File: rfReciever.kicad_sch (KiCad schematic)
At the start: 27 parts, among them P1 USB_C_Plug_USB2.0, SW1 SW_Push, SW2 SW_Push, U1 XBee_SMT, U2 CP2102N-Axx-xQFN20, U3 USBLC6-2SC6

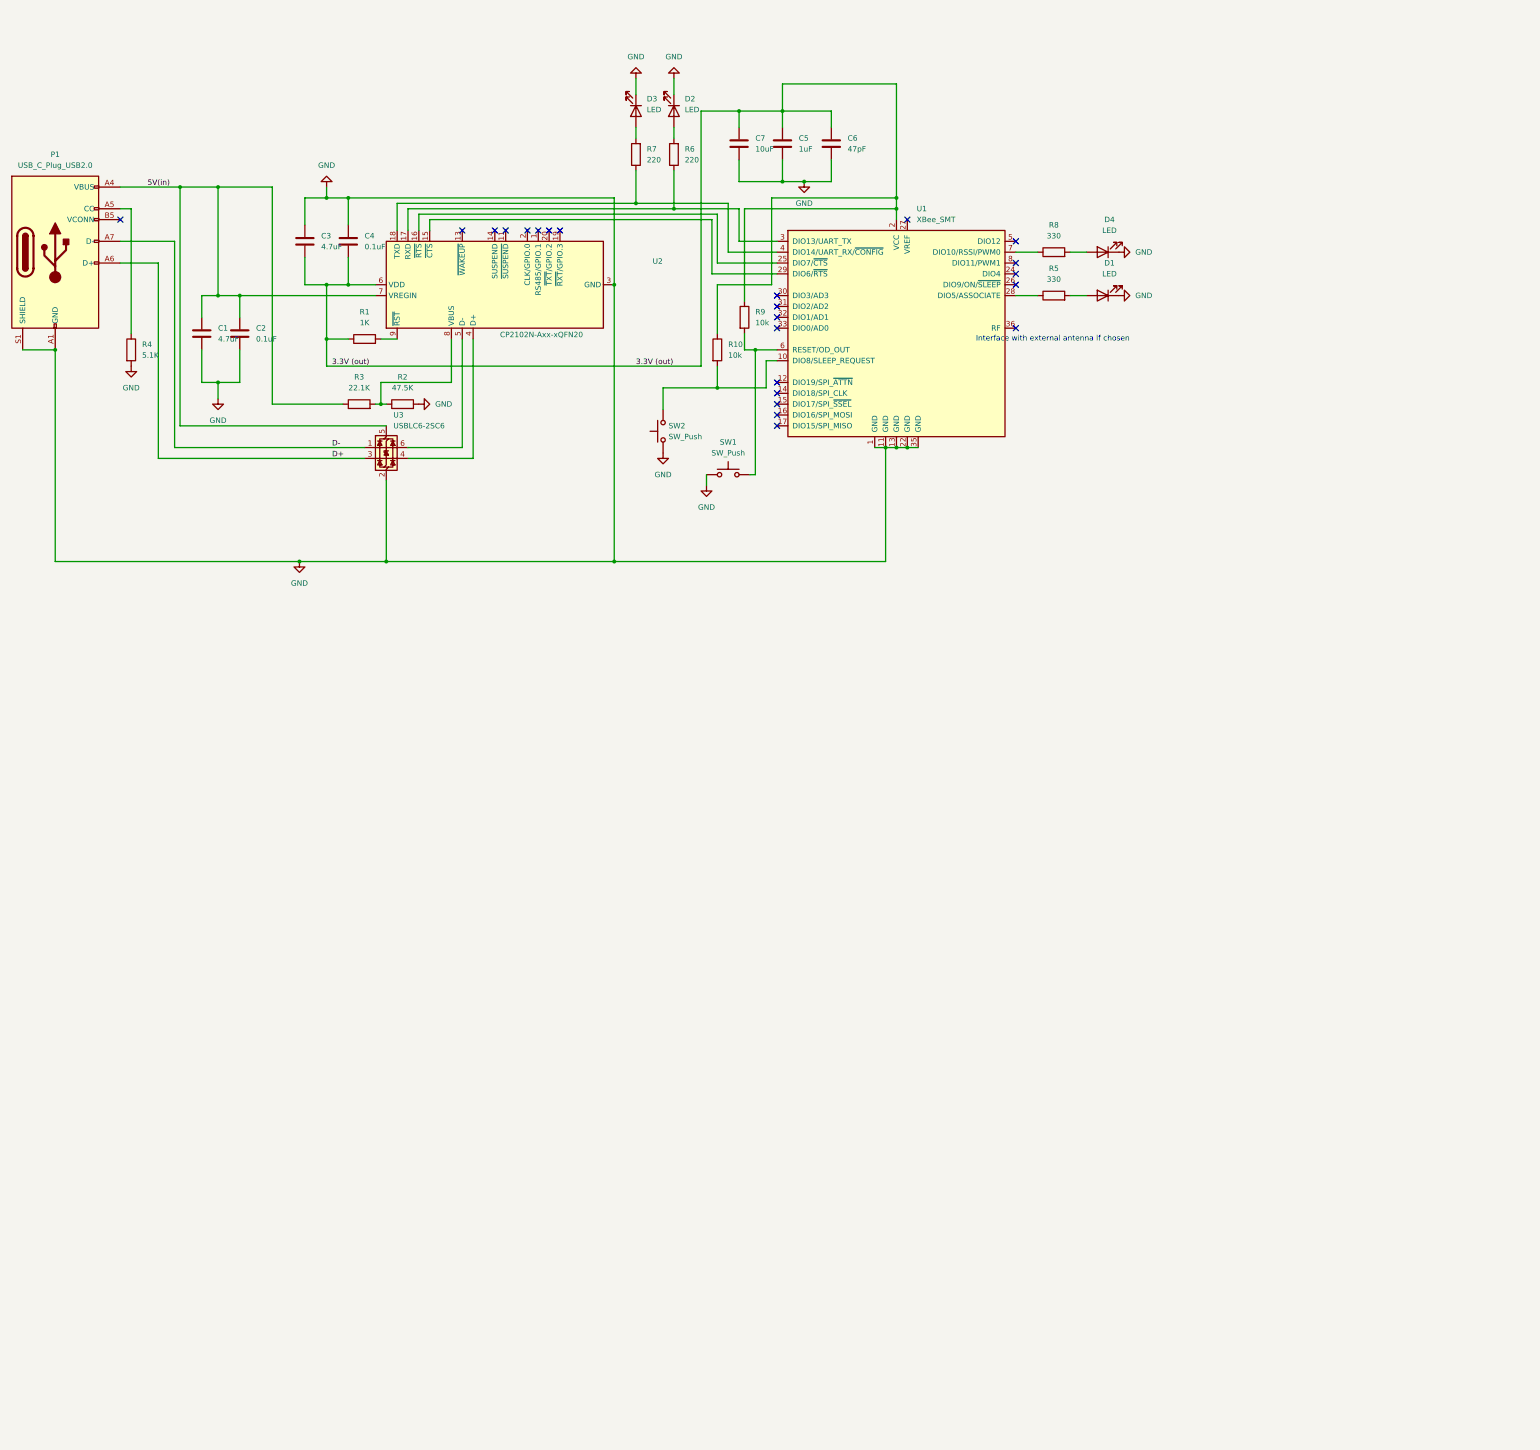
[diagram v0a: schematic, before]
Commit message: double schematic about to fix
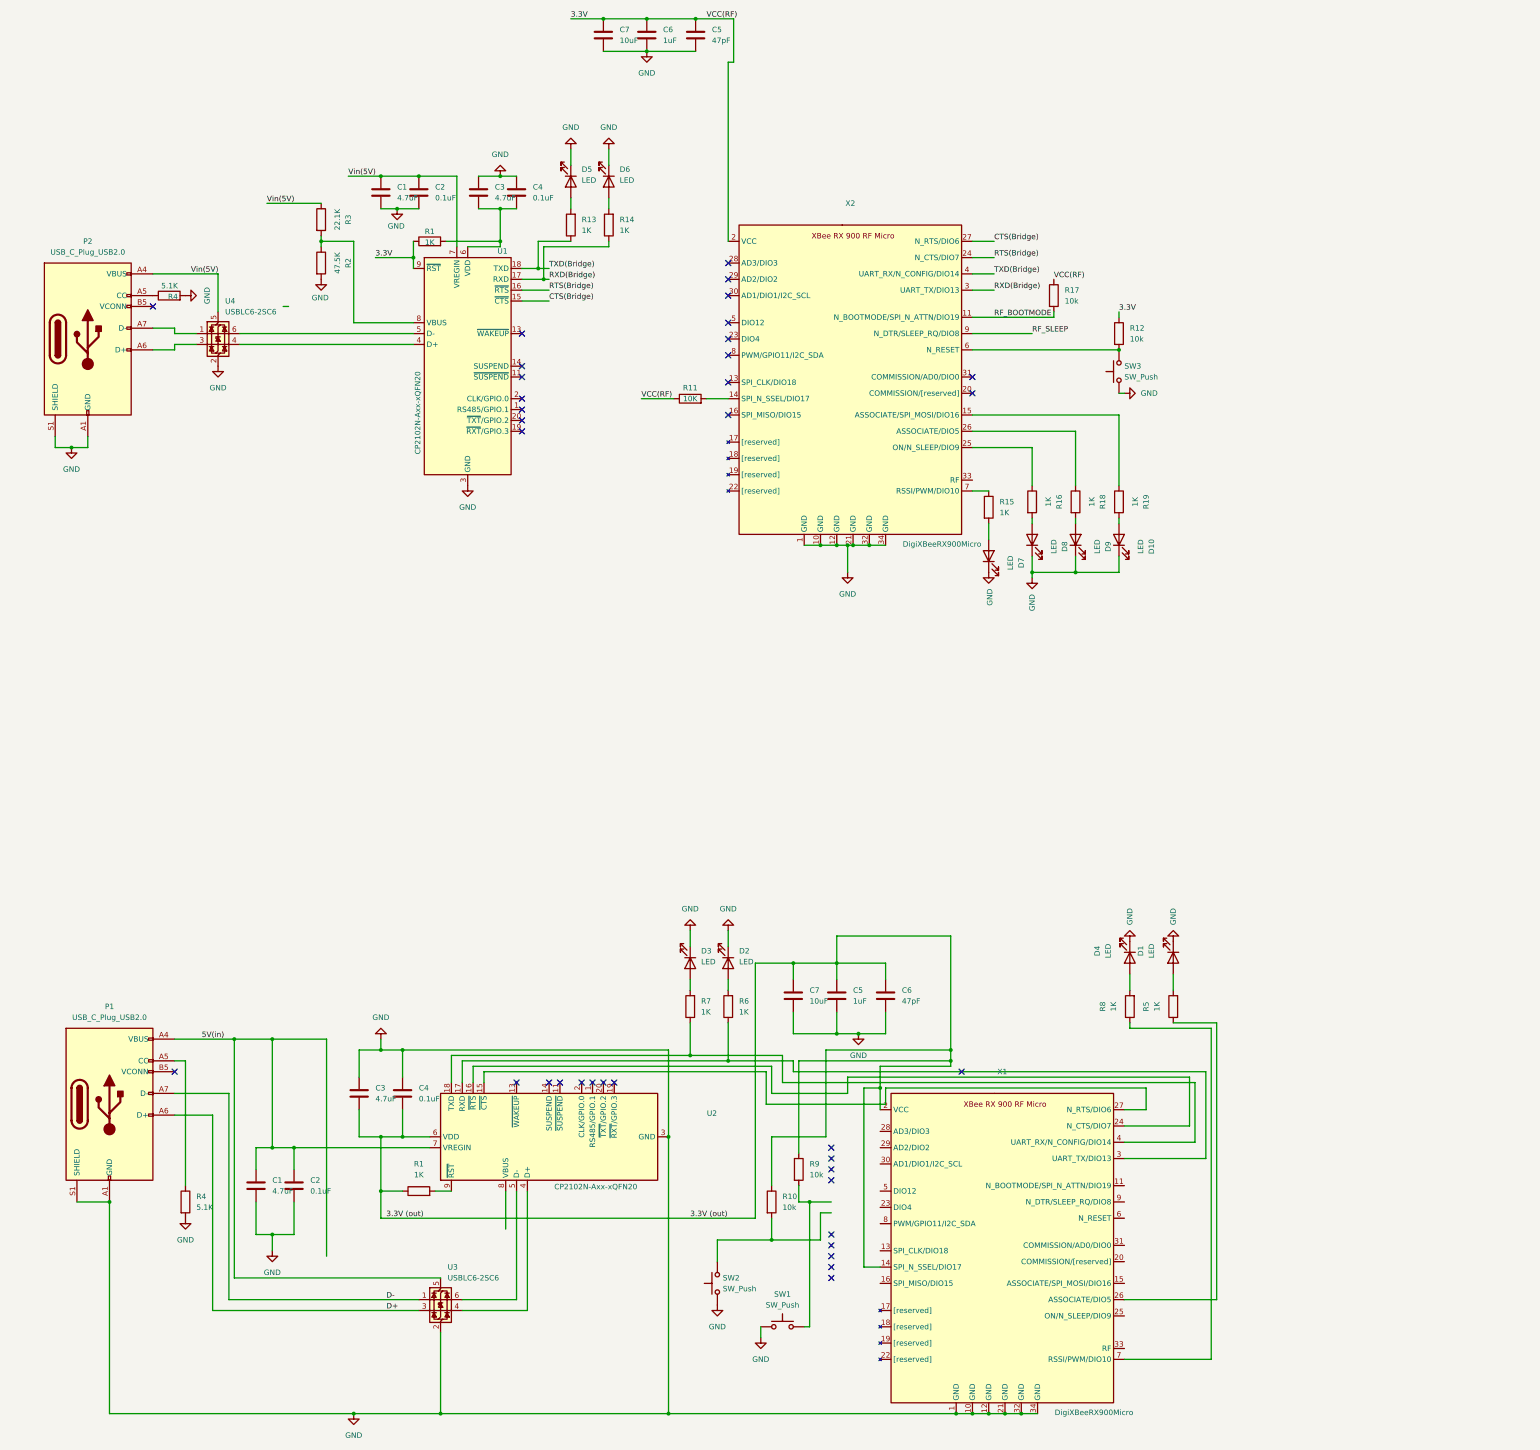
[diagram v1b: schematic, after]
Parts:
- removed U1: XBee_SMT, RF_Module:Digi_XBee_SMT, symbol RF_ZigBee:XBee_SMT
- added C1, C3: 4.7uF, Capacitor_SMD:C_0805_2012Metric, symbol Device:C
- added C2, C4: 0.1uF, Capacitor_SMD:C_0805_2012Metric, symbol Device:C
- added C5: 47pF, Capacitor_SMD:C_0805_2012Metric, symbol Device:C
- added C6: 1uF, Capacitor_SMD:C_0805_2012Metric, symbol Device:C
- added C7: 10uF, Capacitor_SMD:C_0805_2012Metric, symbol Device:C
- added D10, D5, D6, D7, D8, D9: LED, LED_SMD:LED_0805_2012Metric, symbol Device:LED
- added P2: USB_C_Plug_USB2.0, Connector_USB:USB_C_Plug_JAE_DX07P024AJ1, symbol Connector:USB_C_Plug_USB2.0
- added R1, R13, R14, R15, R16, R18, R19: 1K, Resistor_SMD:R_0805_2012Metric, symbol Device:R
- added R11: 10K, Resistor_SMD:R_0805_2012Metric, symbol Device:R
- added R12, R17: 10k, Resistor_SMD:R_0805_2012Metric, symbol Device:R
- added R4: 5.1K, Resistor_SMD:R_0805_2012Metric, symbol Device:R
- added SW3: SW_Push, Button_Switch_THT:SW_PUSH_6mm_H4.3mm, symbol Switch:SW_Push
- added U1: CP2102N-Axx-xQFN20, Audio_Module:QFN24_CP2102N_SIL, symbol Interface_USB:CP2102N-Axx-xQFN20
- added U4: USBLC6-2SC6, Package_TO_SOT_SMD:SOT-23-6, symbol Power_Protection:USBLC6-2SC6
- added X1, X2: DigiXBeeRX900Micro, symbol DataAcqLeaderBoard-Symbols:DigiXBeeRX900Micro
- C1, C3, C5: footprint Capacitor_SMD:C_0603_1608Metric_Pad1.08x0.95mm_HandSolder -> Capacitor_SMD:C_0805_2012Metric
- C2: footprint Capacitor_SMD:C_01005_0402Metric_Pad0.57x0.30mm_HandSolder -> Capacitor_SMD:C_0805_2012Metric
- C4, C6: footprint Capacitor_SMD:C_0402_1005Metric_Pad0.74x0.62mm_HandSolder -> Capacitor_SMD:C_0805_2012Metric
- C7: footprint Capacitor_SMD:C_0805_2012Metric_Pad1.18x1.45mm_HandSolder -> Capacitor_SMD:C_0805_2012Metric
- D1, D4: footprint LED_SMD:LED_0201_0603Metric -> LED_SMD:LED_0805_2012Metric
- D2, D3: footprint LED_SMD:LED_0603_1608Metric_Pad1.05x0.95mm_HandSolder -> LED_SMD:LED_0805_2012Metric
- R1, R10, R2, R3, R4, R9: footprint Resistor_SMD:R_0603_1608Metric_Pad0.98x0.95mm_HandSolder -> Resistor_SMD:R_0805_2012Metric
- R5, R8: value 330 -> 1K; footprint Resistor_SMD:R_0603_1608Metric_Pad0.98x0.95mm_HandSolder -> Resistor_SMD:R_0805_2012Metric
- R6, R7: value 220 -> 1K; footprint Resistor_SMD:R_0603_1608Metric_Pad0.98x0.95mm_HandSolder -> Resistor_SMD:R_0805_2012Metric
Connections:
- net 3.3V (out): now also X1.14 (SPI_N_SSEL/DIO17), X1.2 (VCC)
- net 5V(in): no longer R3.1
- net GND: now also C1.2, C2.2, C3.1, C4.1, C5.2, C6.2, C7.2, D10.1 (K), D5.1 (K), D6.1 (K), D7.1 (K), D8.1 (K), D9.1 (K), P2.A1 (GND), P2.A12 (GND), P2.B1 (GND), P2.B12 (GND), P2.S1 (SHIELD), R4.2, SW3.1, U1.12 (GND), U1.21 (GND), U1.3 (GND), U4.2 (GND), X1.1 (GND), X1.10 (GND), X1.12 (GND), X1.21 (GND), X1.32 (GND), X1.34 (GND), X2.1 (GND), X2.10 (GND), X2.12 (GND), X2.21 (GND), X2.32 (GND), X2.34 (GND)
- net at R2.1, R3.2: now also U1.8 (VBUS); no longer U2.8 (VBUS)
- net at R7.1, U2.18 (TXD): now also X1.4 (UART_RX/N_CONFIG/DIO14)
- net at R6.1, U2.17 (RXD): now also X1.3 (UART_TX/DIO13)
- net at R8.1: now also X1.7 (RSSI/PWM/DIO10)
- net at R5.1: now also X1.26 (ASSOCIATE/DIO5)
- net at U2.16 (~{RTS}): now also X1.24 (N_CTS/DIO7)
- net at U2.15 (~{CTS}): now also X1.27 (N_RTS/DIO6)
- new net: D6.2 (A), R14.2
- new net: C3.2, C4.2, R1.2, U1.6 (VDD)
- new net: P2.A5 (CC), R4.1
- new net: R19.1, X2.15 (ASSOCIATE/SPI_MOSI/DIO16)
- new net: D10.2 (A), R19.2
- new net: R12.2, SW3.2, X2.6 (N_RESET)
- new net: R11.2, X2.14 (SPI_N_SSEL/DIO17)
- new net: D5.2 (A), R13.2
- new net: R16.1, X2.25 (ON/N_SLEEP/DIO9)
- new net: R18.1, X2.26 (ASSOCIATE/DIO5)
- new net: R15.1, X2.7 (RSSI/PWM/DIO10)
- new net: D7.2 (A), R15.2
- new net: D8.2 (A), R16.2
- new net: D9.2 (A), R18.2
- new net: P2.A6 (D+), U4.3 (I/O2)
- new net: P2.A7 (D-), U4.1 (I/O1)
- new net: U1.4 (D+), U4.4 (I/O2)
- new net: U1.5 (D-), U4.6 (I/O1)
- new net 3.3V: C5.1, C6.1, C7.1, R1.1, R11.1, R12.1, R17.1, U1.9 (~{RST}), X2.2 (VCC)
- new net CTS(Bridge): U1.15 (~{CTS}), X2.27 (N_RTS/DIO6)
- new net RF_BOOTMODE: R17.2, X2.11 (N_BOOTMODE/SPI_N_ATTN/DIO19)
- new net RF_SLEEP: X2.9 (N_DTR/SLEEP_RQ/DIO8)
- new net RTS(Bridge): U1.16 (~{RTS}), X2.24 (N_CTS/DIO7)
- new net RXD(Bridge): R14.1, U1.17 (RXD), X2.3 (UART_TX/DIO13)
- new net TXD(Bridge): R13.1, U1.18 (TXD), X2.4 (UART_RX/N_CONFIG/DIO14)
- new net Vin(5V): C1.1, C2.1, P2.A4 (VBUS), P2.A9 (VBUS), P2.B4 (VBUS), P2.B9 (VBUS), R3.1, U1.7 (VREGIN), U4.5 (VBUS)
- no-connect marks 23 -> 36
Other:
- note removed: "Interface with external antenna if chosen"
- moved on the sheet: C1, C2, C3, C4, C5, C6, C7, D1, D2, D3, D4, P1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

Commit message: Final Schematic preliminary pcb layout(pre-routing)
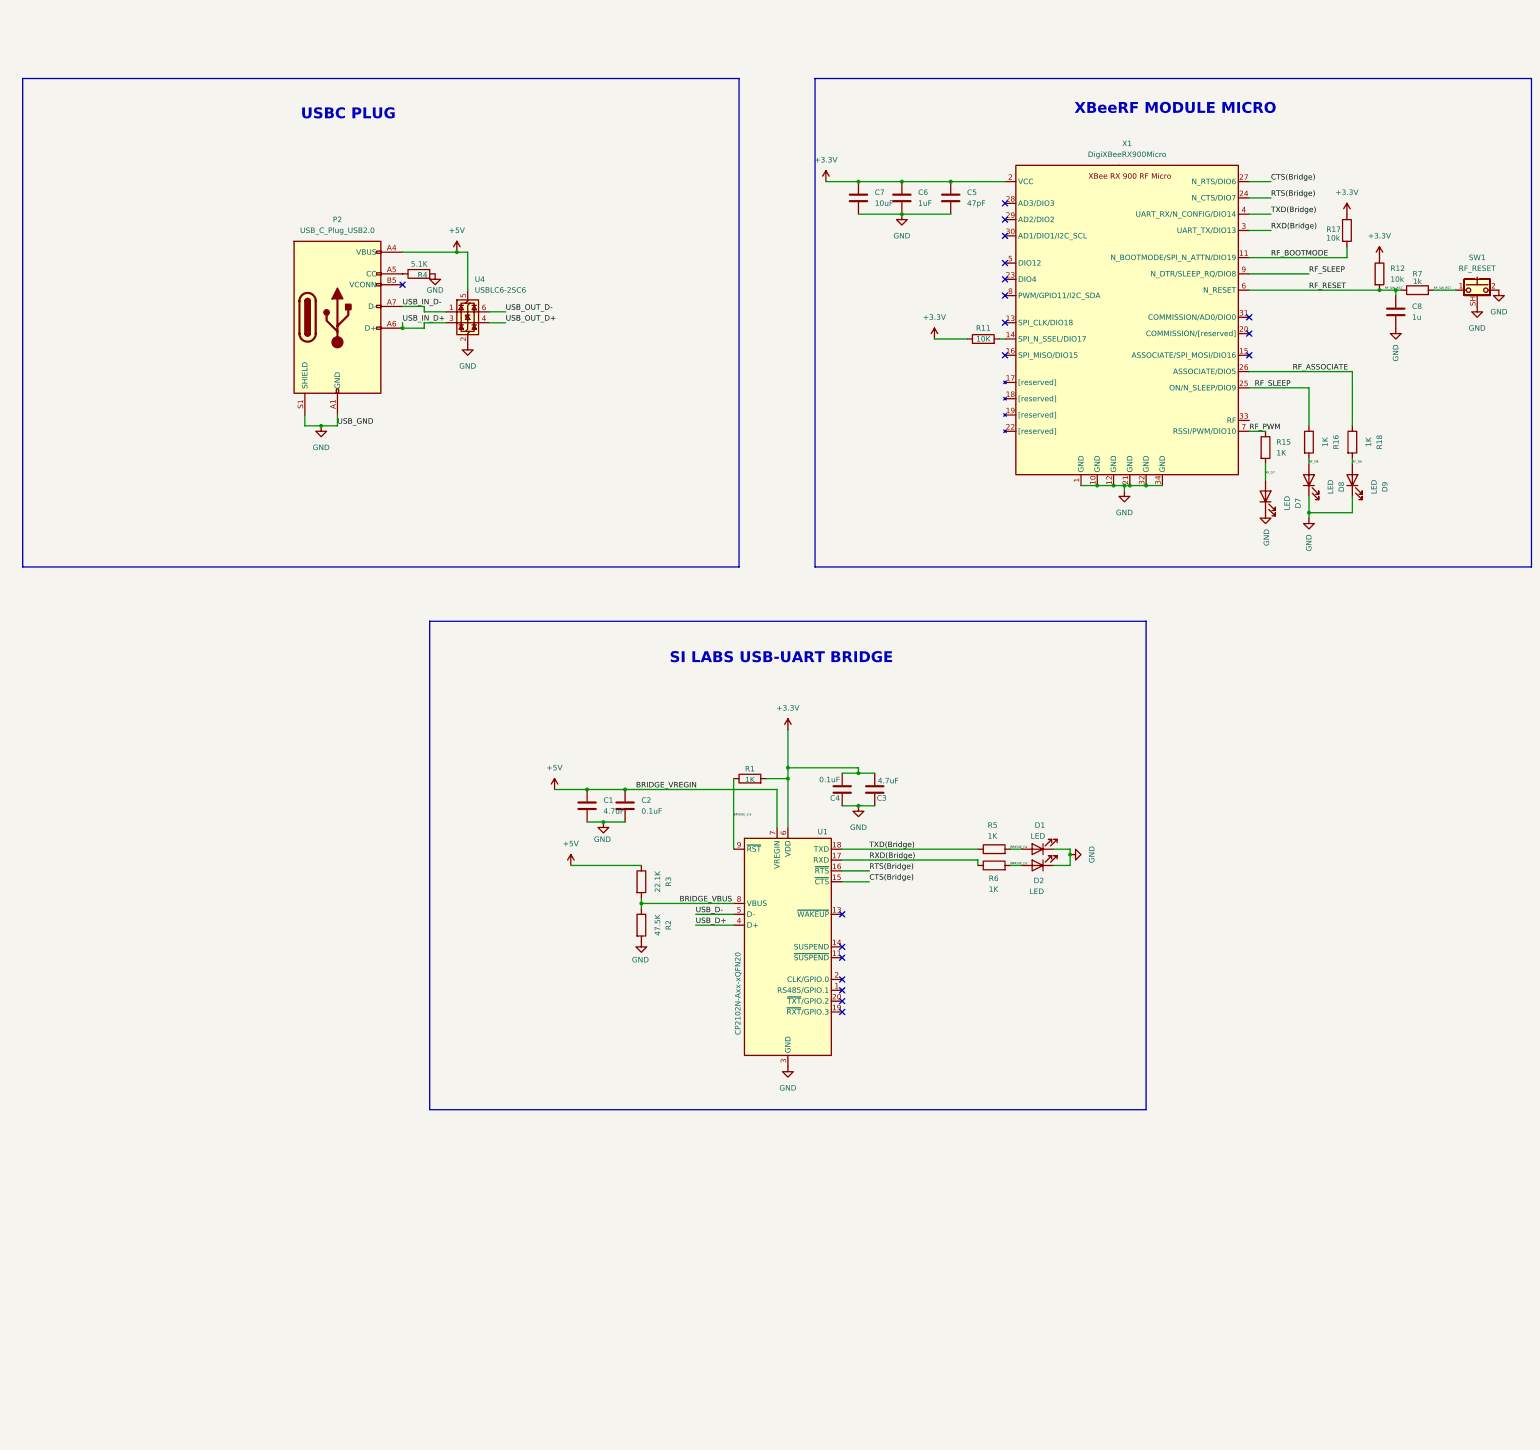
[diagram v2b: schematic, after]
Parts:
- removed C1, C3: 4.7uF, Capacitor_SMD:C_0805_2012Metric, symbol Device:C
- removed C2, C4: 0.1uF, Capacitor_SMD:C_0805_2012Metric, symbol Device:C
- removed C5: 1uF, Capacitor_SMD:C_0805_2012Metric, symbol Device:C
- removed C6: 47pF, Capacitor_SMD:C_0805_2012Metric, symbol Device:C
- removed C7: 10uF, Capacitor_SMD:C_0805_2012Metric, symbol Device:C
- removed D10, D3, D4, D5, D6: LED, LED_SMD:LED_0805_2012Metric, symbol Device:LED
- removed P1: USB_C_Plug_USB2.0, Connector_USB:USB_C_Plug_JAE_DX07P024AJ1, symbol Connector:USB_C_Plug_USB2.0
- removed R1, R13, R14, R19, R8: 1K, Resistor_SMD:R_0805_2012Metric, symbol Device:R
- removed R10, R9: 10k, Resistor_SMD:R_0805_2012Metric, symbol Device:R
- removed R4: 5.1K, Resistor_SMD:R_0805_2012Metric, symbol Device:R
- removed SW1, SW2, SW3: SW_Push, Button_Switch_THT:SW_PUSH_6mm_H4.3mm, symbol Switch:SW_Push
- removed U2: CP2102N-Axx-xQFN20, Audio_Module:QFN24_CP2102N_SIL, symbol Interface_USB:CP2102N-Axx-xQFN20
- removed U3: USBLC6-2SC6, Package_TO_SOT_SMD:SOT-23-6, symbol Power_Protection:USBLC6-2SC6
- removed X1, X2: DigiXBeeRX900Micro, symbol DataAcqLeaderBoard-Symbols:DigiXBeeRX900Micro
- added C8: 1u, Capacitor_SMD:C_0805_2012Metric, symbol Device:C
- added SW1: RF_RESET, Button_Switch_SMD:SW_SPST_CK_KMS2xxGP, symbol Switch:CK_KMS2xxG
- added X1: DigiXBeeRX900Micro, rfReciever-Footprints:XBeeXR900RFMicro, symbol xBeeRFSymbol:DigiXBeeRX900Micro
- R7: value 1K -> 1k; Link (none) -> https://www.mouser.com/ProductDetail/Vishay-Dale/CRCW08051K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; Mouser Part Number (none) -> 71-CRCW08051K00FKEAC; P/N (none) -> CRCW08051K00FKEAC
- U1: footprint Audio_Module:QFN24_CP2102N_SIL -> rfReciever-Footprints:QFN50P500X500X80-29N
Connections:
- net CTS(Bridge): now also X1.27 (N_RTS/DIO6)
- net GND: now also C8.2, SW1.2, SW1.SH (B), X1.1 (GND), X1.10 (GND), X1.12 (GND), X1.21 (GND), X1.32 (GND), X1.34 (GND)
- net RF_BOOTMODE: now also X1.11 (N_BOOTMODE/SPI_N_ATTN/DIO19)
- net RF_SLEEP: now also R16.1, X1.25 (ON/N_SLEEP/DIO9), X1.9 (N_DTR/SLEEP_RQ/DIO8)
- net RTS(Bridge): now also X1.24 (N_CTS/DIO7)
- net RXD(Bridge): now also R6.1, X1.3 (UART_TX/DIO13)
- net TXD(Bridge): now also R5.1, X1.4 (UART_RX/N_CONFIG/DIO14)
- net BRIDGE_VBUS: now reaches R2.1, R3.2, U1.8 (VBUS)
- net +3.3V: now reaches C3.2, C4.2, R1.2, U1.6 (VDD)
- net +3.3V: now also C5.1, C6.1, C7.1, R11.1, R12.1, R17.1, X1.2 (VCC)
- net BRIDGE_D1: now reaches D1.2 (A), R5.2
- net RF_RESET: now reaches R7.1
- net RF_RESET: now also R12.2, R7.2, C8.1, SW1.1, X1.6 (N_RESET)
- net BRIDGE_D2: now reaches D2.2 (A), R6.2
- net at R11.2: now also X1.14 (SPI_N_SSEL/DIO17)
- net RF_ASSOCIATE: now reaches R18.1
- net RF_ASSOCIATE: now also X1.26 (ASSOCIATE/DIO5)
- net RF_PWM: now reaches R15.1
- net RF_PWM: now also X1.7 (RSSI/PWM/DIO10)
- net RF_D7: now reaches D7.2 (A), R15.2
- net RF_D8: now reaches D8.2 (A), R16.2
- net RF_D9: now reaches D9.2 (A), R18.2
- net USB_IN_D+: now reaches P2.A6 (D+), U4.3 (I/O2)
- net USB_IN_D-: now reaches P2.A7 (D-), U4.1 (I/O1)
- net USB_D+: now reaches U1.4 (D+)
- net USB_D+: no longer U4.4 (I/O2)
- net USB_D-: now reaches U1.5 (D-)
- net USB_D-: no longer U4.6 (I/O1)
- removed net 3.3V: C5.1, C6.1, C7.1, R1.1, R11.1, R12.1, R17.1, U1.9 (~{RST})
- net Vin(5V) renamed +5V
- new net BRIDGE_3.3: R1.1, U1.9 (~{RST})
- new net USB_OUT_D+: U4.4 (I/O2)
- new net USB_OUT_D-: U4.6 (I/O1)
- no-connect marks 36 -> 19
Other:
- note added: "SI LABS USB-UART BRIDGE"
- note added: "USBC PLUG"
- note added: "XBeeRF MODULE MICRO"
- moved on the sheet: C1, C2, C3, C4, C5, C6, C7, D7, D8, D9, P2, R1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
